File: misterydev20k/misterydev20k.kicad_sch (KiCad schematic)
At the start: 45 parts, among them J1 SWD, J2 USB_C_Receptacle_USB2.0, SW1 SW_Push, U1 XC6206PxxxMR-Regulator_Linear, U2 W25Q128JVS, U3 USBLC6-2SC6, U4 RP2040, Y1 12MHz

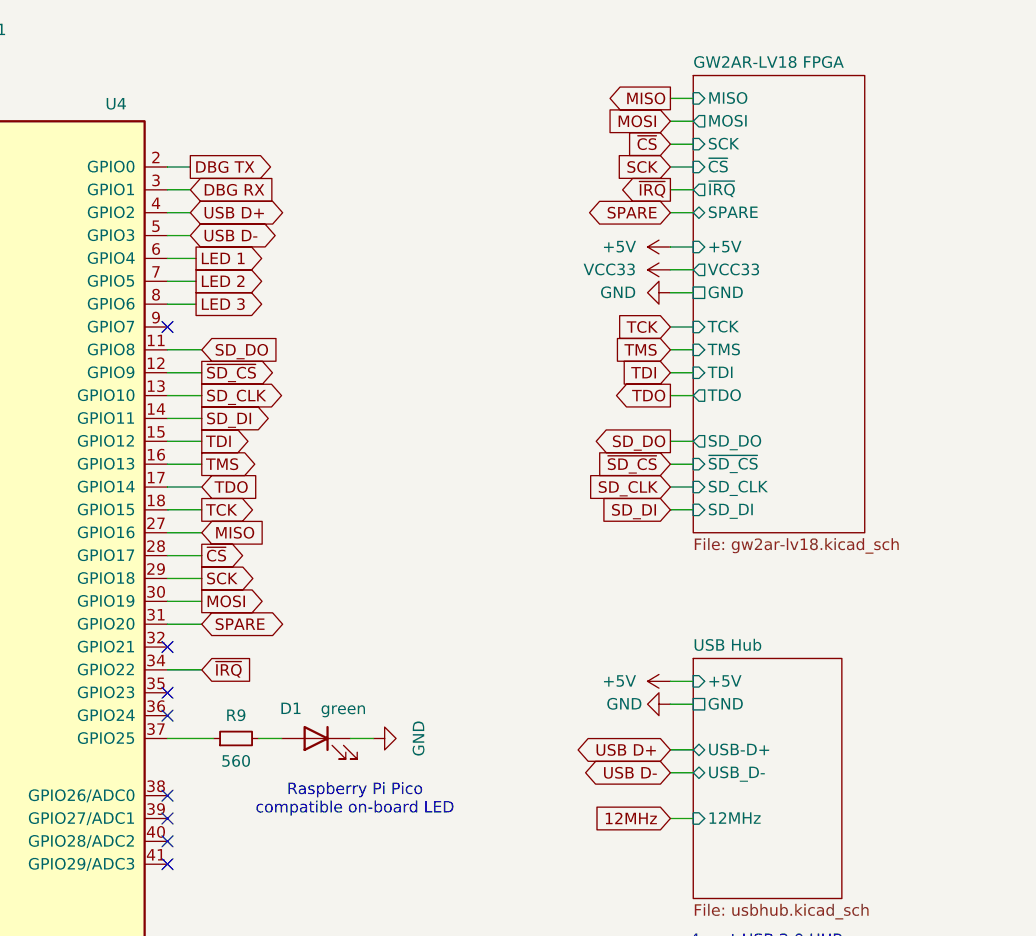
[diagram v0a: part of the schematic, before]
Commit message: Some dev board progress
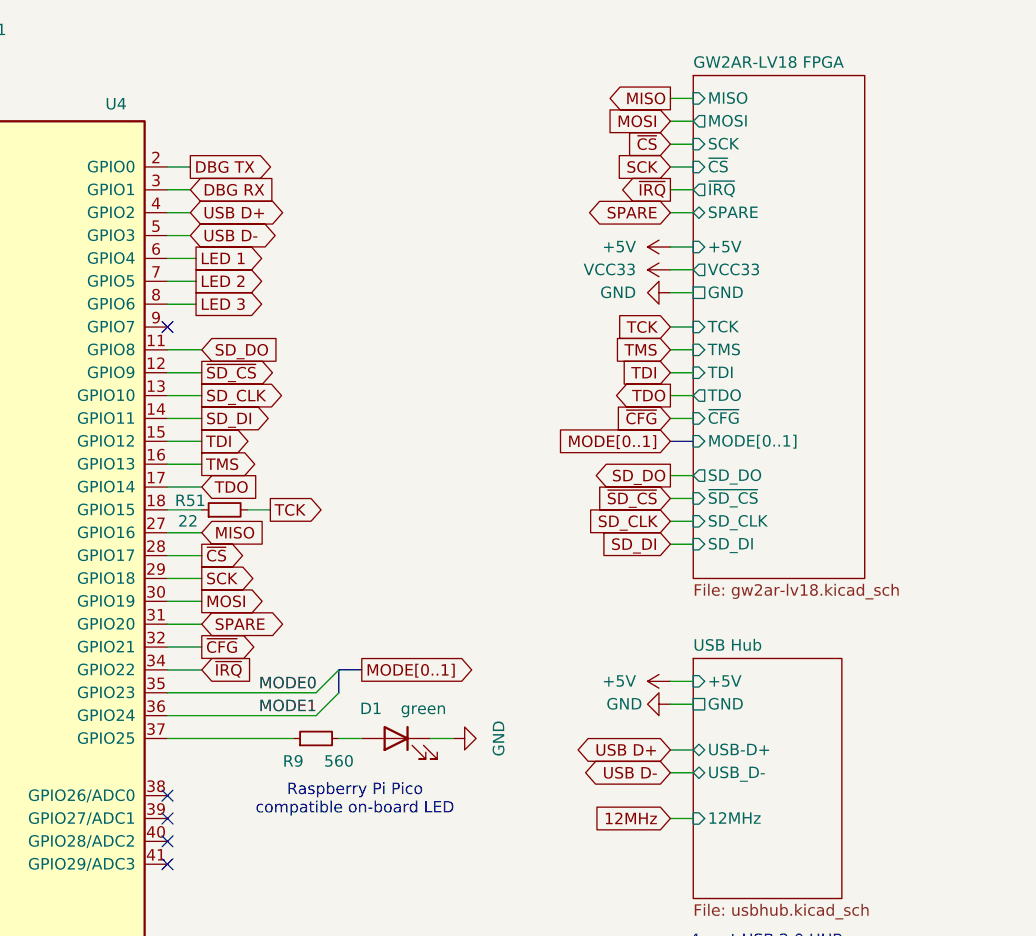
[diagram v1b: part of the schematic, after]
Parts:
- added R51: 22, Resistor_SMD:R_0402_1005Metric, symbol Device:R_Small
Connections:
- net TCK: now also R51.2; no longer U4.18 (GPIO15)
- net ~{CFG}: now reaches U4.32 (GPIO21)
- net MODE0: now reaches U4.35 (GPIO23)
- net MODE1: now reaches U4.36 (GPIO24)
- new net: R51.1, U4.18 (GPIO15)
- no-connect marks 10 -> 7
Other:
- sheet GW2AR-LV18 FPGA ports: added MODE[0..1], ~{CFG}; removed none
- moved on the sheet: D1, R9
